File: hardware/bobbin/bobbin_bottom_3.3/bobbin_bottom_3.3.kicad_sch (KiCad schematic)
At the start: 2 parts, among them J1 Conn_01x01, J2 Conn_01x03

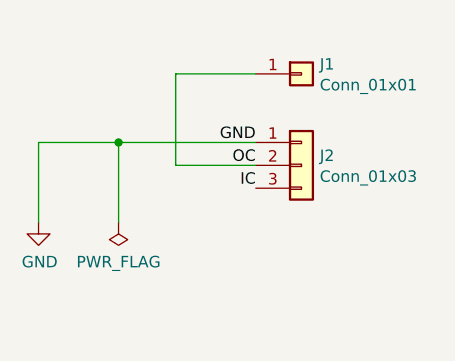
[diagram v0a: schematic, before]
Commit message: First shot v2 bobbin for 3.3"
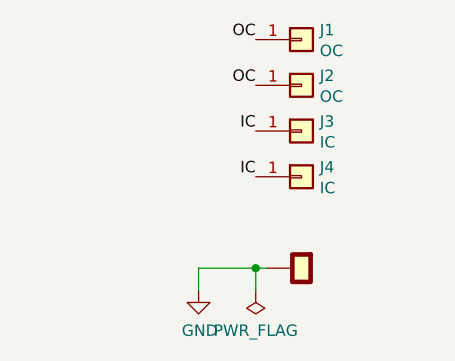
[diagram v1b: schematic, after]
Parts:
- removed J2: Conn_01x03, cycfi_library:xr2-coil-connector, symbol Connector_Generic:Conn_01x03
- added H1: single_pad, xr_spectra_library:rail_slot_3.3, symbol cycfi_library:single_pad
- added J1: OC, cycfi_library:single-pad-1.52x1.52-th, symbol Connector_Generic:Conn_01x01
- added J3, J4: IC, cycfi_library:single-pad-1.52x1.52-th, symbol Connector_Generic:Conn_01x01
- J2: renamed from J1; value Conn_01x01 -> OC; footprint cycfi_library:xr2-oc-coil-connector -> cycfi_library:single-pad-1.52x1.52-th
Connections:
- net GND: now also H1.1
- net IC: now also J3.1 (Pin_1), J4.1 (Pin_1)
- net OC: now also J1.1 (Pin_1)
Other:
- moved on the sheet: J2
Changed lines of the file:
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@@
 (kicad_sch (version 20211123) (generator eeschema)
   (paper "A4")
-  (junction (at 132.08 67.31) (diameter 0) (color 0 0 0 0)
+  (junction (at 147.32 81.28) (diameter 0) (color 0 0 0 0)
   )
-  (wire (pts (xy 132.08 67.31) (xy 132.08 76.2))
+  (wire (pts (xy 140.97 81.28) (xy 147.32 81.28))
     (stroke (width 0) (type default) (color 0 0 0 0))
   )
-  (wire (pts (xy 147.32 69.85) (xy 138.43 69.85))
+  (wire (pts (xy 140.97 81.28) (xy 140.97 83.82))
     (stroke (width 0) (type default) (color 0 0 0 0))
   )
-  (wire (pts (xy 123.19 67.31) (xy 123.19 76.2))
+  (wire (pts (xy 147.32 81.28) (xy 147.32 83.82))
     (stroke (width 0) (type default) (color 0 0 0 0))
   )
-  (wire (pts (xy 132.08 67.31) (xy 147.32 67.31))
+  (wire (pts (xy 147.32 81.28) (xy 148.59 81.28))
     (stroke (width 0) (type default) (color 0 0 0 0))
   )
-  (wire (pts (xy 138.43 69.85) (xy 138.43 59.69))
-    (stroke (width 0) (type default) (color 0 0 0 0))
-  )
-  (wire (pts (xy 123.19 67.31) (xy 132.08 67.31))
-    (stroke (width 0) (type default) (color 0 0 0 0))
-  )
-  (wire (pts (xy 138.43 59.69) (xy 147.32 59.69))
-    (stroke (width 0) (type default) (color 0 0 0 0))
-  )
-  (label "GND" (at 147.32 67.31 180)
+  (label "IC" (at 147.32 71.12 180)
     (effects (font (size 1.27 1.27)) (justify right bottom))
   )
-  (label "OC" (at 147.32 69.85 180)
+  (label "OC" (at 147.32 60.96 180)
     (effects (font (size 1.27 1.27)) (justify right bottom))
   )
-  (label "IC" (at 147.32 72.39 180)
+  (label "OC" (at 147.32 55.88 180)
     (effects (font (size 1.27 1.27)) (justify right bottom))
   )
-  (symbol (lib_id "power:GND") (at 123.19 76.2 0) (unit 1)
+  (label "IC" (at 147.32 66.04 180)
+    (effects (font (size 1.27 1.27)) (justify right bottom))
+  )
+  (symbol (lib_id "Connector_Generic:Conn_01x01") (at 152.4 60.96 0) (unit 1)
     (in_bom yes) (on_board yes)
-    (property "Reference" "#PWR01" (id 0) (at 123.19 82.55 0)
+    (property "Reference" "J2" (id 0) (at 154.432 59.8932 0)
+      (effects (font (size 1.27 1.27)) (justify left))
+    )
+    (property "Value" "OC" (id 1) (at 154.432 62.2046 0)
+      (effects (font (size 1.27 1.27)) (justify left))
+    )
+    (property "Footprint" "cycfi_library:single-pad-1.52x1.52-th" (id 2) (at 152.4 60.96 0)
       (effects (font (size 1.27 1.27)) hide)
     )
-    (property "Value" "GND" (id 1) (at 123.317 80.5942 0))
-    (property "Footprint" "" (id 2) (at 123.19 76.2 0)
-      (effects (font (size 1.27 1.27)) hide)
-    )
-    (property "Datasheet" "" (id 3) (at 123.19 76.2 0)
+    (property "Datasheet" "~" (id 3) (at 152.4 60.96 0)
       (effects (font (size 1.27 1.27)) hide)
     )
     (pin "1")
   )
-  (symbol (lib_id "power:PWR_FLAG") (at 132.08 76.2 180) (unit 1)
+  (symbol (lib_id "power:GND") (at 140.97 83.82 0) (unit 1)
     (in_bom yes) (on_board yes)
-    (property "Reference" "#FLG01" (id 0) (at 132.08 78.105 0)
+    (property "Reference" "#PWR01" (id 0) (at 140.97 90.17 0)
       (effects (font (size 1.27 1.27)) hide)
     )
-    (property "Value" "PWR_FLAG" (id 1) (at 132.08 80.5942 0))
-    (property "Footprint" "" (id 2) (at 132.08 76.2 0)
+    (property "Value" "GND" (id 1) (at 141.097 88.2142 0))
+    (property "Footprint" "" (id 2) (at 140.97 83.82 0)
       (effects (font (size 1.27 1.27)) hide)
     )
-    (property "Datasheet" "~" (id 3) (at 132.08 76.2 0)
+    (property "Datasheet" "" (id 3) (at 140.97 83.82 0)
       (effects (font (size 1.27 1.27)) hide)
     )
     (pin "1")
   )
-  (symbol (lib_id "Connector_Generic:Conn_01x01") (at 152.4 59.69 0) (unit 1)
+  (symbol (lib_id "power:PWR_FLAG") (at 147.32 83.82 180) (unit 1)
     (in_bom yes) (on_board yes)
-    (property "Reference" "J1" (id 0) (at 154.432 58.6232 0)
-      (effects (font (size 1.27 1.27)) (justify left))
-    )
-    (property "Value" "Conn_01x01" (id 1) (at 154.432 60.9346 0)
-      (effects (font (size 1.27 1.27)) (justify left))
-    )
-    (property "Footprint" "cycfi_library:xr2-oc-coil-connector" (id 2) (at 152.4 59.69 0)
+    (property "Reference" "#FLG01" (id 0) (at 147.32 85.725 0)
       (effects (font (size 1.27 1.27)) hide)
     )
-    (property "Datasheet" "~" (id 3) (at 152.4 59.69 0)
+    (property "Value" "PWR_FLAG" (id 1) (at 147.32 88.2142 0))
+    (property "Footprint" "" (id 2) (at 147.32 83.82 0)
+      (effects (font (size 1.27 1.27)) hide)
+    )
+    (property "Datasheet" "~" (id 3) (at 147.32 83.82 0)
       (effects (font (size 1.27 1.27)) hide)
     )
     (pin "1")
   )
-  (symbol (lib_id "Connector_Generic:Conn_01x03") (at 152.4 69.85 0) (unit 1)
+  (symbol (lib_id "cycfi_library:single_pad") (at 151.13 81.28 270) (unit 1)
     (in_bom yes) (on_board yes)
-    (property "Reference" "J2" (id 0) (at 154.432 68.7832 0)
-      (effects (font (size 1.27 1.27)) (justify left))
+    (property "Reference" "H1" (id 0) (at 154.305 81.28 0)
+      (effects (font (size 1.27 1.27)) (justify left) hide)
     )
-    (property "Value" "Conn_01x03" (id 1) (at 154.432 71.0946 0)
-      (effects (font (size 1.27 1.27)) (justify left))
-    )
-    (property "Footprint" "cycfi_library:xr2-coil-connector" (id 2) (at 152.4 69.85 0)
+    (property "Value" "single_pad" (id 1) (at 156.21 81.28 0)
       (effects (font (size 1.27 1.27)) hide)
     )
-    (property "Datasheet" "~" (id 3) (at 152.4 69.85 0)
+    (property "Footprint" "xr_spectra_library:rail_slot_3.3" (id 2) (at 151.13 81.28 0)
+      (effects (font (size 1.27 1.27)) hide)
+    )
+    (property "Datasheet" "~" (id 3) (at 151.13 81.28 0)
       (effects (font (size 1.27 1.27)) hide)
     )
     (pin "1")
-    (pin "2")
-    (pin "3")
+  )
+  (symbol (lib_id "Connector_Generic:Conn_01x01") (at 152.4 55.88 0) (unit 1)
+    (in_bom yes) (on_board yes)
+    (property "Reference" "J1" (id 0) (at 154.432 54.8132 0)
+      (effects (font (size 1.27 1.27)) (justify left))
+    )
+    (property "Value" "OC" (id 1) (at 154.432 57.1246 0)
+      (effects (font (size 1.27 1.27)) (justify left))
+    )
+    (property "Footprint" "cycfi_library:single-pad-1.52x1.52-th" (id 2) (at 152.4 55.88 0)
+      (effects (font (size 1.27 1.27)) hide)
+    )
+    (property "Datasheet" "~" (id 3) (at 152.4 55.88 0)
+      (effects (font (size 1.27 1.27)) hide)
+    )
+    (pin "1")
+  )
+  (symbol (lib_id "Connector_Generic:Conn_01x01") (at 152.4 71.12 0) (unit 1)
+    (in_bom yes) (on_board yes)
+    (property "Reference" "J4" (id 0) (at 154.432 70.0532 0)
+      (effects (font (size 1.27 1.27)) (justify left))
+    )
+    (property "Value" "IC" (id 1) (at 154.432 72.3646 0)
+      (effects (font (size 1.27 1.27)) (justify left))
+    )
+    (property "Footprint" "cycfi_library:single-pad-1.52x1.52-th" (id 2) (at 152.4 71.12 0)
+      (effects (font (size 1.27 1.27)) hide)
+    )
+    (property "Datasheet" "~" (id 3) (at 152.4 71.12 0)
+      (effects (font (size 1.27 1.27)) hide)
+    )
+    (pin "1")
+  )
+  (symbol (lib_id "Connector_Generic:Conn_01x01") (at 152.4 66.04 0) (unit 1)
+    (in_bom yes) (on_board yes)
+    (property "Reference" "J3" (id 0) (at 154.432 64.9732 0)
+      (effects (font (size 1.27 1.27)) (justify left))
+    )
+    (property "Value" "IC" (id 1) (at 154.432 67.2846 0)
+      (effects (font (size 1.27 1.27)) (justify left))
+    )
+    (property "Footprint" "cycfi_library:single-pad-1.52x1.52-th" (id 2) (at 152.4 66.04 0)
+      (effects (font (size 1.27 1.27)) hide)
+    )
+    (property "Datasheet" "~" (id 3) (at 152.4 66.04 0)
+      (effects (font (size 1.27 1.27)) hide)
+    )
+    (pin "1")
   )
   (sheet_instances
@@
   )
   (symbol_instances
-    (path "/00000000-0000-0000-0000-000060d8ce57"
+    (path "/2af67c9f-1758-4649-8401-6b678ded3579"
       (reference "#FLG01") (unit 1) (value "PWR_FLAG") (footprint "")
     )
-    (path "/00000000-0000-0000-0000-000060d88df5"
+    (path "/01d2f9bc-2a40-45e2-aace-1a8287a77613"
       (reference "#PWR01") (unit 1) (value "GND") (footprint "")
     )
+    (path "/56a51644-b55f-492b-aa38-d2c3e210984a"
+      (reference "H1") (unit 1) (value "single_pad") (footprint "xr_spectra_library:rail_slot_3.3")
+    )
+    (path "/9ed5f09d-f428-462b-978c-7a9dd8637c06"
+      (reference "J1") (unit 1) (value "OC") (footprint "cycfi_library:single-pad-1.52x1.52-th")
+    )
     (path "/00000000-0000-0000-0000-00006150ec9c"
-      (reference "J1") (unit 1) (value "Conn_01x01") (footprint "cycfi_library:xr2-oc-coil-connector")
+      (reference "J2") (unit 1) (value "OC") (footprint "cycfi_library:single-pad-1.52x1.52-th")
     )
-    (path "/00000000-0000-0000-0000-0000615174b9"
-      (reference "J2") (unit 1) (value "Conn_01x03") (footprint "cycfi_library:xr2-coil-connector")
+    (path "/f226d0fa-6fa6-4f46-99cf-6860d539dd2c"
+      (reference "J3") (unit 1) (value "IC") (footprint "cycfi_library:single-pad-1.52x1.52-th")
+    )
+    (path "/a996384d-e545-45bd-921b-60bec151aabf"
+      (reference "J4") (unit 1) (value "IC") (footprint "cycfi_library:single-pad-1.52x1.52-th")
     )
   )
